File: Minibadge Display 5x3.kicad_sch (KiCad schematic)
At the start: 2 parts, among them J4 Conn_02x05_Odd_Even

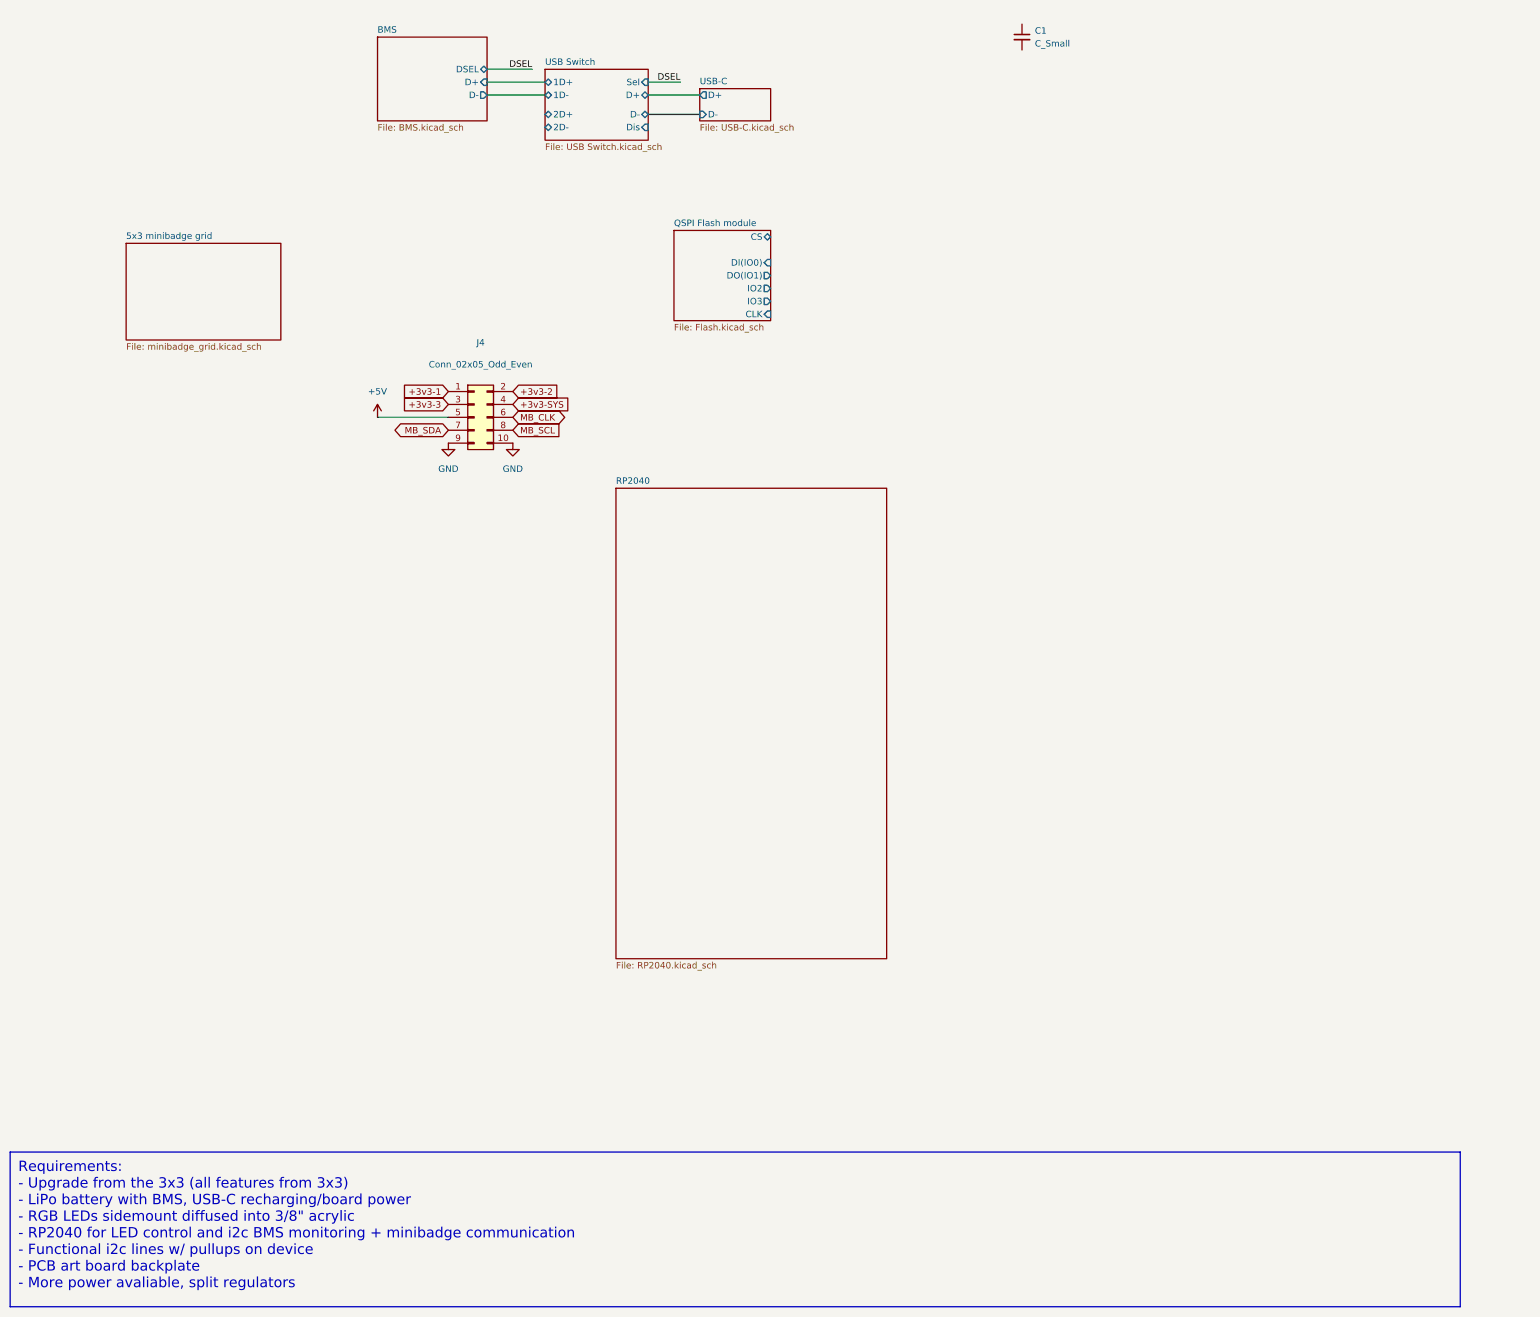
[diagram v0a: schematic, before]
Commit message: more rp2040 work
-BMS updates
- rp2040 updates
- add hardware design docs
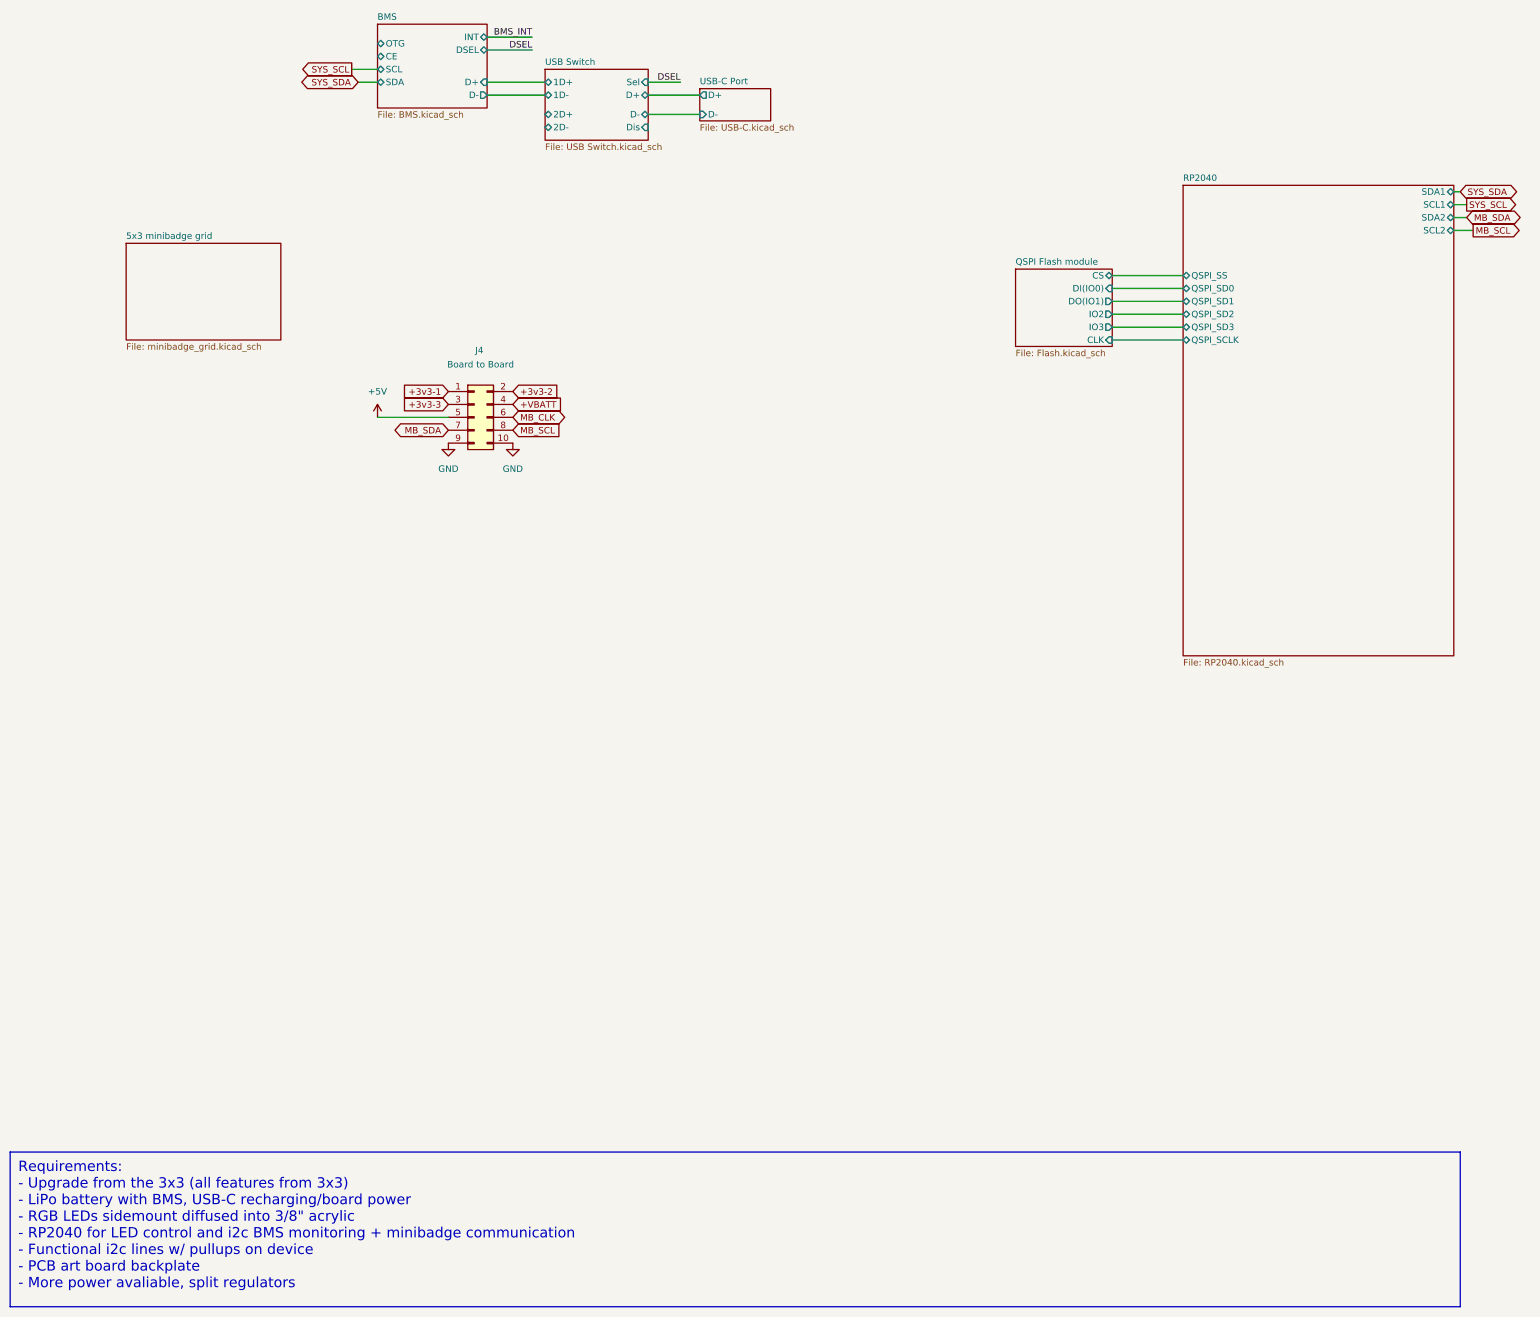
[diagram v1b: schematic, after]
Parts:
- removed C1: C_Small, symbol Device:C_Small
- J4: value Conn_02x05_Odd_Even -> Board to Board
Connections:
- net +3v3-SYS renamed +VBATT
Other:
- sheet USB-C renamed USB-C Port
- sheet BMS ports: added CE, INT, OTG, SCL, SDA; removed none
- sheet RP2040 ports: added QSPI_SCLK, QSPI_SD0, QSPI_SD1, QSPI_SD2, QSPI_SD3, QSPI_SS, SCL1, SCL2, SDA1, SDA2; removed none
